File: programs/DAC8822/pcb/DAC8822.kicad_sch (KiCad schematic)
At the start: 22 parts, among them J1 TFT ST7735, J2 Conn_01x04_Pin, J3 Conn_01x04_Pin, J4 Screw_Terminal_01x02, J5 Conn_01x04_Pin, J6 Conn_01x04_Pin, U1 8BVG4, U2 8BVG4, U3 RP2350B-WeAct, U4 OPA2277, U5 OPA2277, U6 OPA2277, U7 OPA2277, U8 LM7805

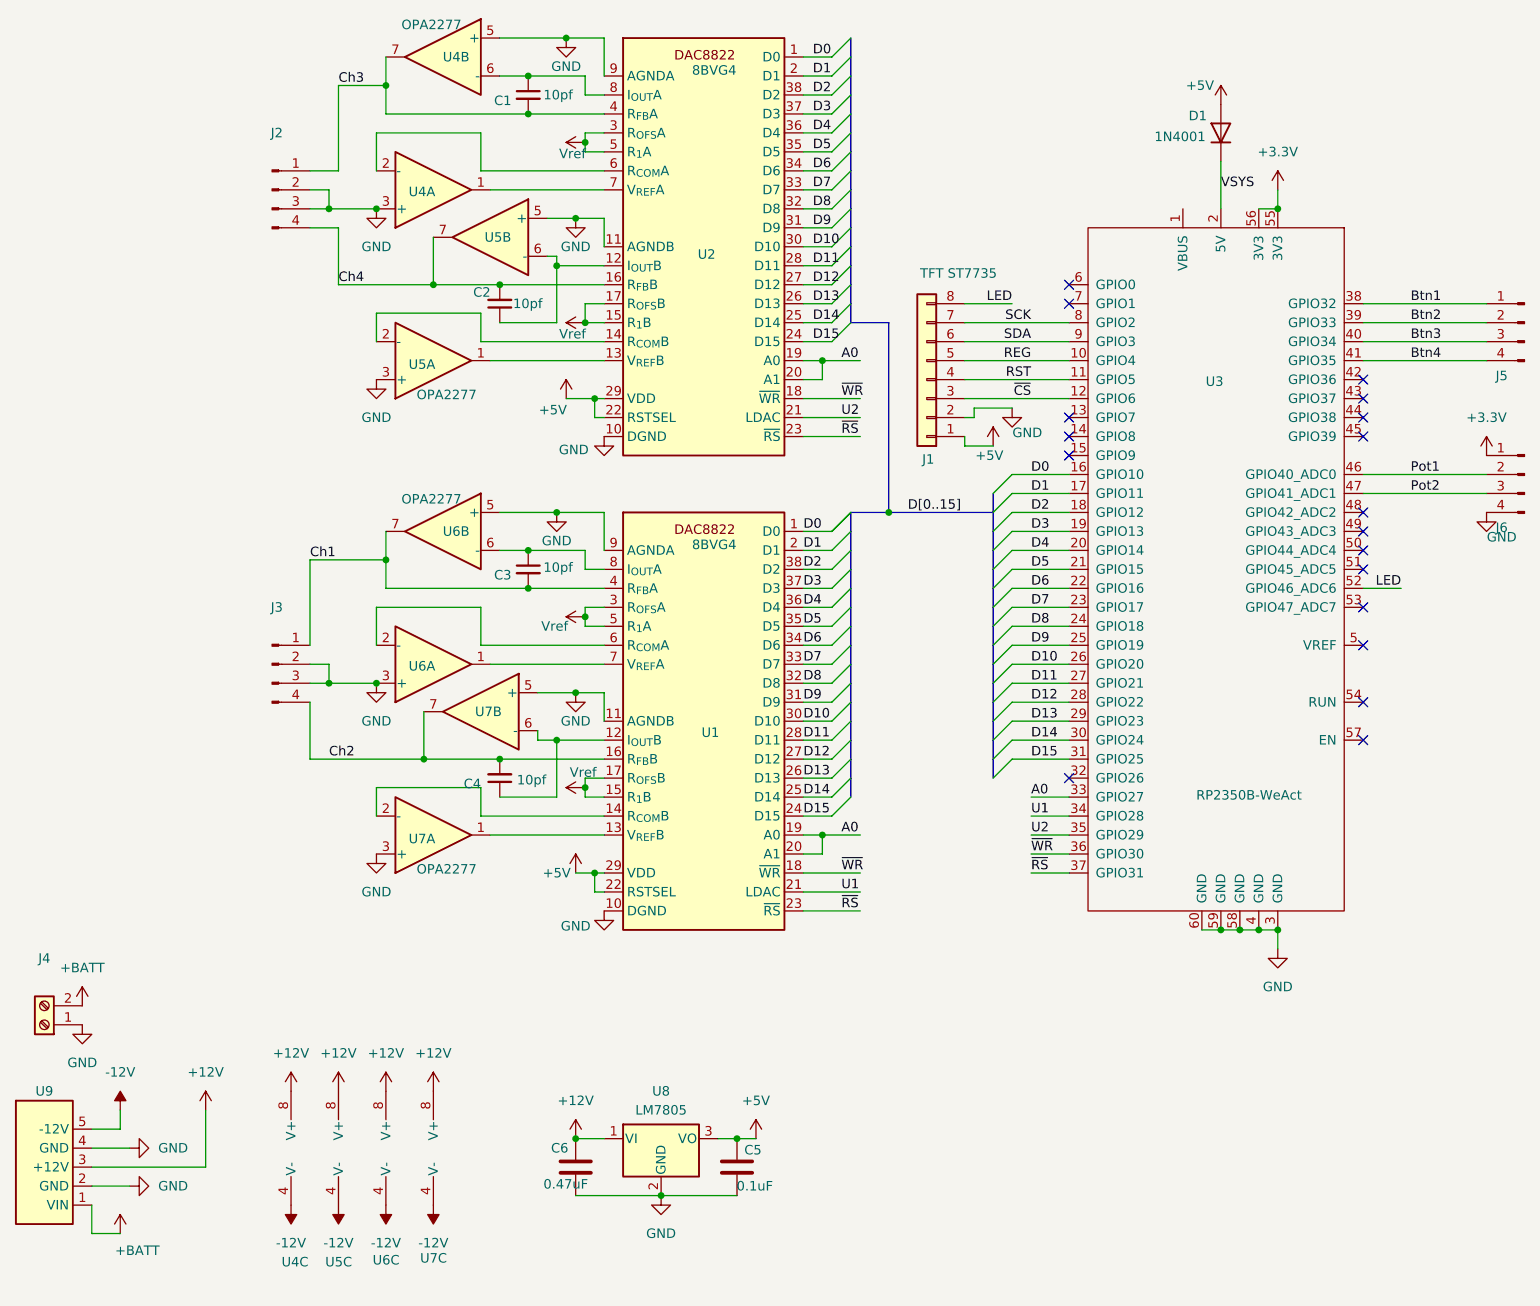
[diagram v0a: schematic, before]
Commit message: Add files via upload
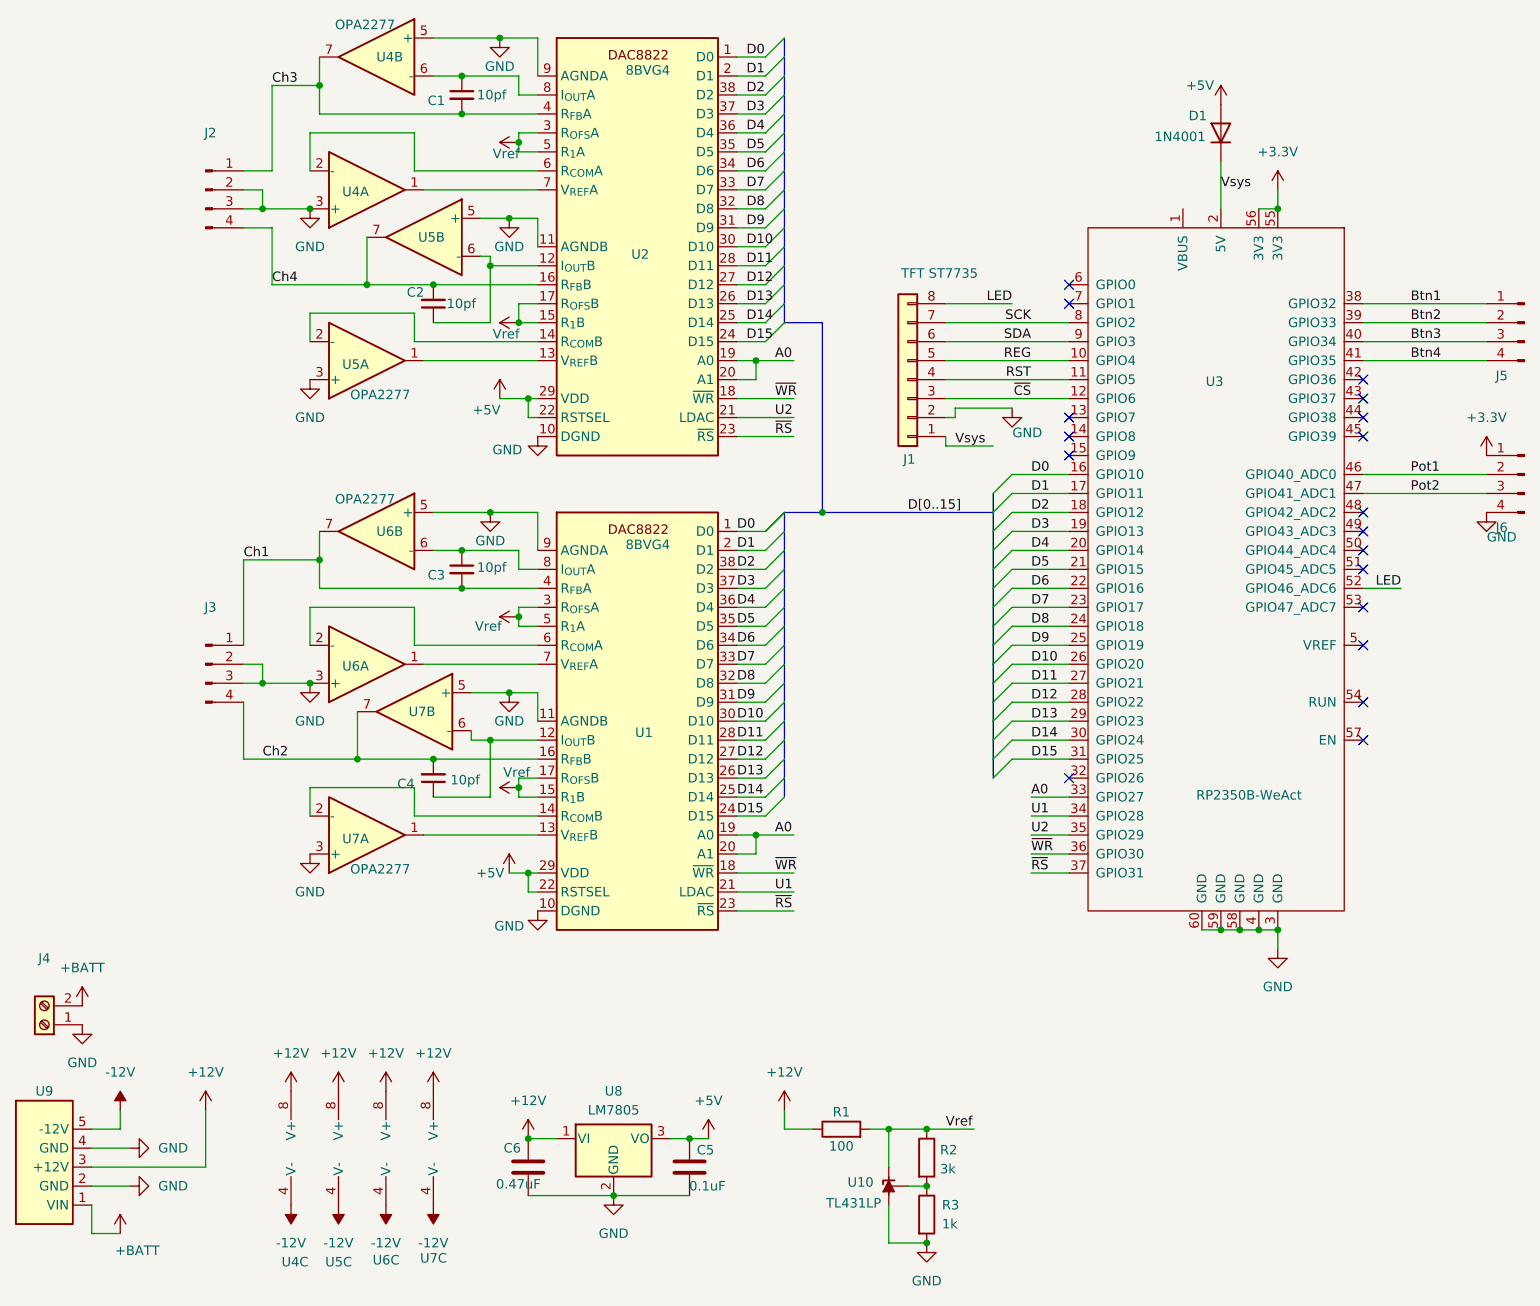
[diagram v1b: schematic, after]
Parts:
- added R1: 100, Resistor_SMD:R_0805_2012Metric, symbol Device:R
- added R2: 3k, Resistor_SMD:R_0805_2012Metric, symbol Device:R
- added R3: 1k, Resistor_SMD:R_0805_2012Metric, symbol Device:R
- added U10: TL431LP, Package_TO_SOT_THT:TO-92_Inline, symbol Reference_Voltage:TL431LP
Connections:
- net +12V: now also R1.1
- net +5V: no longer J1.1 (Pin_1)
- net GND: now also R3.2, U10.2 (A)
- net Vref: now also R1.2, R2.1, U10.3 (K)
- net VSYS renamed Vsys
- net Vsys: now also J1.1 (Pin_1)
- new net: R2.2, R3.1, U10.1 (REF)
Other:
- company: (none) -> Marc Pelletier
- title: (none) -> 4 Ch Signal Generato Pico 2350 and DAC8822 x 2
- moved on the sheet: C1, C2, C3, C4, C5, C6, J1, J2, J3, U1, U2, U4A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

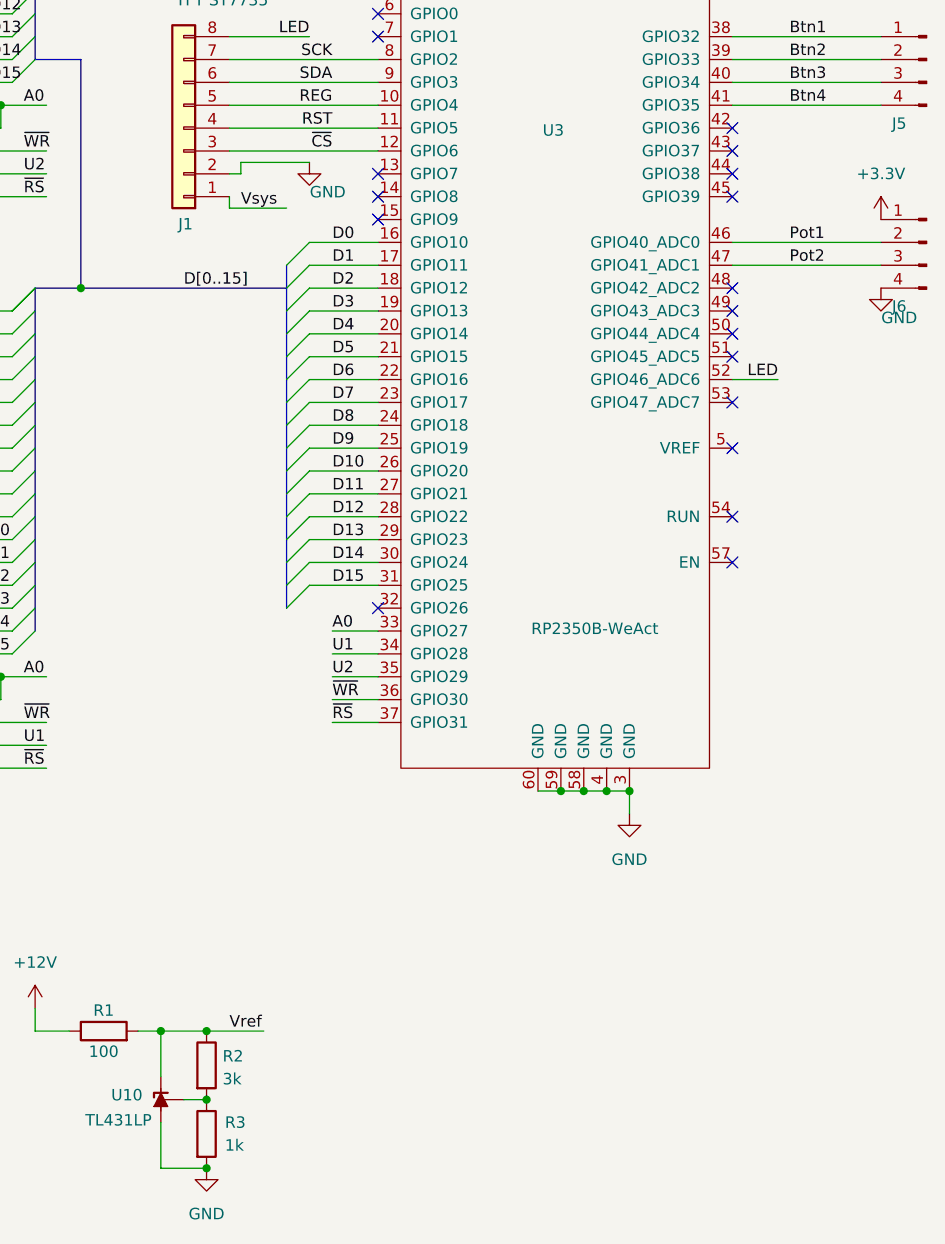
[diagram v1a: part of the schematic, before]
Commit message: Add files via upload
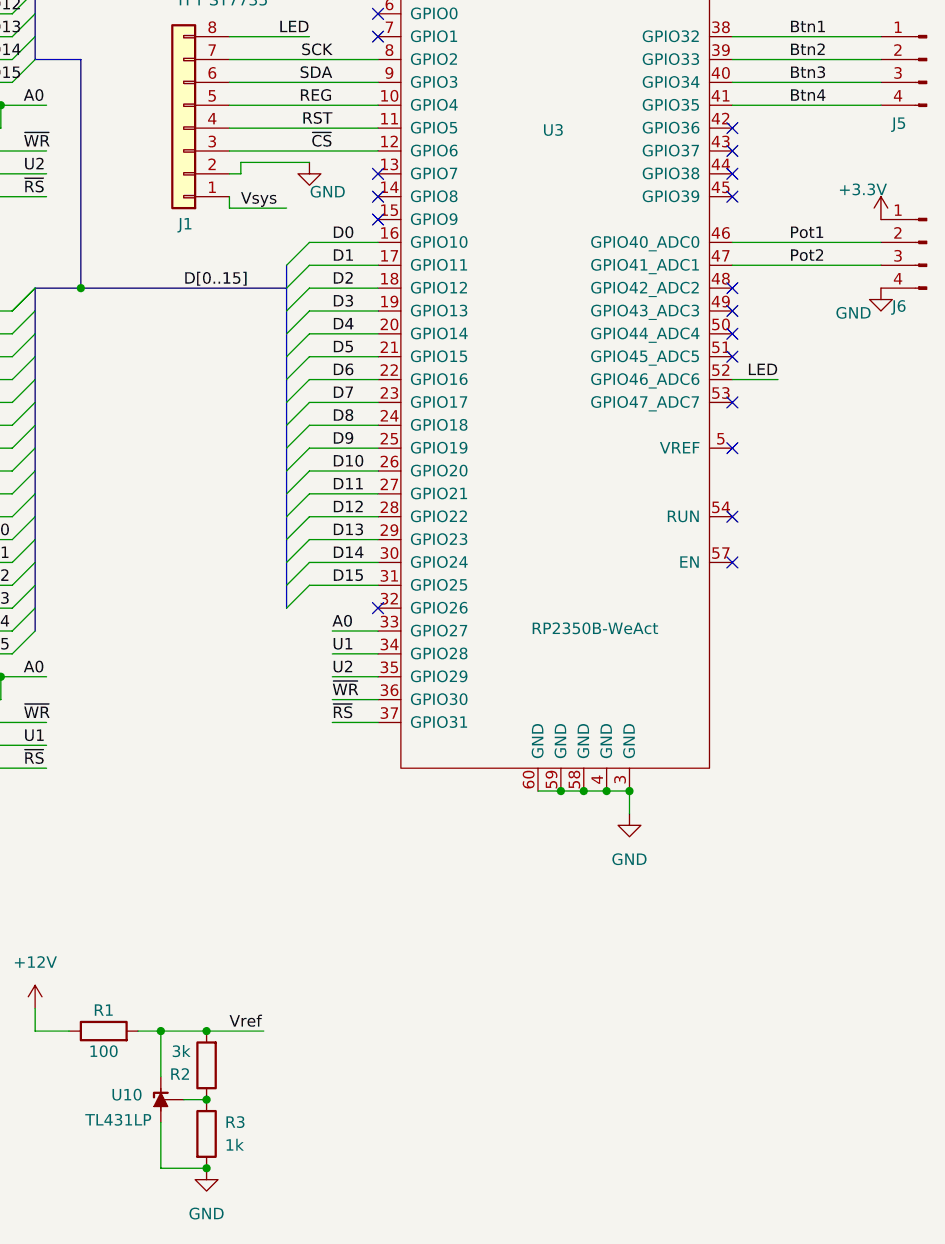
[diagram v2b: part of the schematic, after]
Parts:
- J2, J3, J5, J6: footprint Connector_PinHeader_1.00mm:PinHeader_1x04_P1.00mm_Vertical -> Connector_PinHeader_1.27mm:PinHeader_1x04_P1.27mm_Vertical
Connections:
- net Vref: now also R2.2; no longer R2.1
- net at R3.1, U10.1 (REF): now also R2.1; no longer R2.2
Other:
- moved on the sheet: R2
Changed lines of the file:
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@@
 	)
 	(junction
-		(at 142.24 182.88)
-		(diameter 0)
-		(color 0 0 0 0)
-	)
-	(junction
-		(at 142.24 175.26)
-		(diameter 0)
-		(color 0 0 0 0)
-	)
-	(junction
 		(at 60.96 35.56)
 		(diameter 0)
@@
 	)
 	(junction
+		(at 142.24 175.26)
+		(diameter 0)
+		(color 0 0 0 0)
+	)
+	(junction
 		(at 88.9 176.53)
 		(diameter 0)
@@
 	)
 	(junction
+		(at 142.24 182.88)
+		(diameter 0)
+		(color 0 0 0 0)
+	)
+	(junction
 		(at 59.69 115.57)
 		(diameter 0)
@@
 	(wire
 		(pts
-			(xy 142.24 175.26) (xy 148.59 175.26)
-		)
-		(stroke
-			(width 0)
-			(type default)
-		)
-	)
-	(wire
-		(pts
 			(xy 110.49 176.53) (xy 113.03 176.53)
 		)
@@
 	(wire
 		(pts
+			(xy 142.24 175.26) (xy 148.59 175.26)
+		)
+		(stroke
+			(width 0)
+			(type default)
+		)
+	)
+	(wire
+		(pts
 			(xy 116.84 67.31) (xy 120.65 67.31)
 		)
@@
 			)
 		)
-		(property "Footprint" "Connector_PinHeader_1.00mm:PinHeader_1x04_P1.00mm_Vertical"
+		(property "Footprint" "Connector_PinHeader_1.27mm:PinHeader_1x04_P1.27mm_Vertical"
 			(at 222.25 67.31 0)
 			(effects
@@
 		)
 		(property "Value" "GND"
-			(at 219.202 96.012 0)
+			(at 214.122 95.504 0)
 			(effects
 				(font
@@
 			)
 		)
-		(property "Footprint" "Connector_PinHeader_1.00mm:PinHeader_1x04_P1.00mm_Vertical"
+		(property "Footprint" "Connector_PinHeader_1.27mm:PinHeader_1x04_P1.27mm_Vertical"
 			(at 45.72 49.53 0)
 			(effects
@@
 	(symbol
 		(lib_id "Device:R")
-		(at 142.24 179.07 0)
+		(at 142.24 179.07 180)
 		(unit 1)
 		(exclude_from_sim no)
@@
 		(dnp no)
 		(property "Reference" "R2"
-			(at 144.018 178.054 0)
+			(at 140.462 180.086 0)
 			(effects
 				(font
@@
 		)
 		(property "Value" "3k"
-			(at 144.018 180.594 0)
+			(at 140.462 177.546 0)
 			(effects
 				(font
@@
 		)
 		(property "Footprint" "Resistor_SMD:R_0805_2012Metric"
-			(at 140.462 179.07 90)
+			(at 144.018 179.07 90)
 			(effects
 				(font
@@
 		(on_board yes)
 		(dnp no)
-		(fields_autoplaced yes)
 		(property "Reference" "#PWR040"
 			(at 217.17 88.9 0)
@@
 		)
 		(property "Value" "+3.3V"
-			(at 217.17 80.01 0)
+			(at 215.138 81.788 0)
 			(effects
 				(font
@@
 			)
 		)
-		(property "Footprint" "Connector_PinHeader_1.00mm:PinHeader_1x04_P1.00mm_Vertical"
+		(property "Footprint" "Connector_PinHeader_1.27mm:PinHeader_1x04_P1.27mm_Vertical"
 			(at 45.72 113.03 0)
 			(effects
@@
 			)
 		)
-		(property "Footprint" "Connector_PinHeader_1.00mm:PinHeader_1x04_P1.00mm_Vertical"
+		(property "Footprint" "Connector_PinHeader_1.27mm:PinHeader_1x04_P1.27mm_Vertical"
 			(at 222.25 87.63 0)
 			(effects
